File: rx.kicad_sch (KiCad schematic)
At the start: 49 parts, among them J5 SWH, J7 SMA, J9 SWH, T1 RF_BALUN, T1 RXIF_BALUN, U14 MAX2120, U16 DPDT

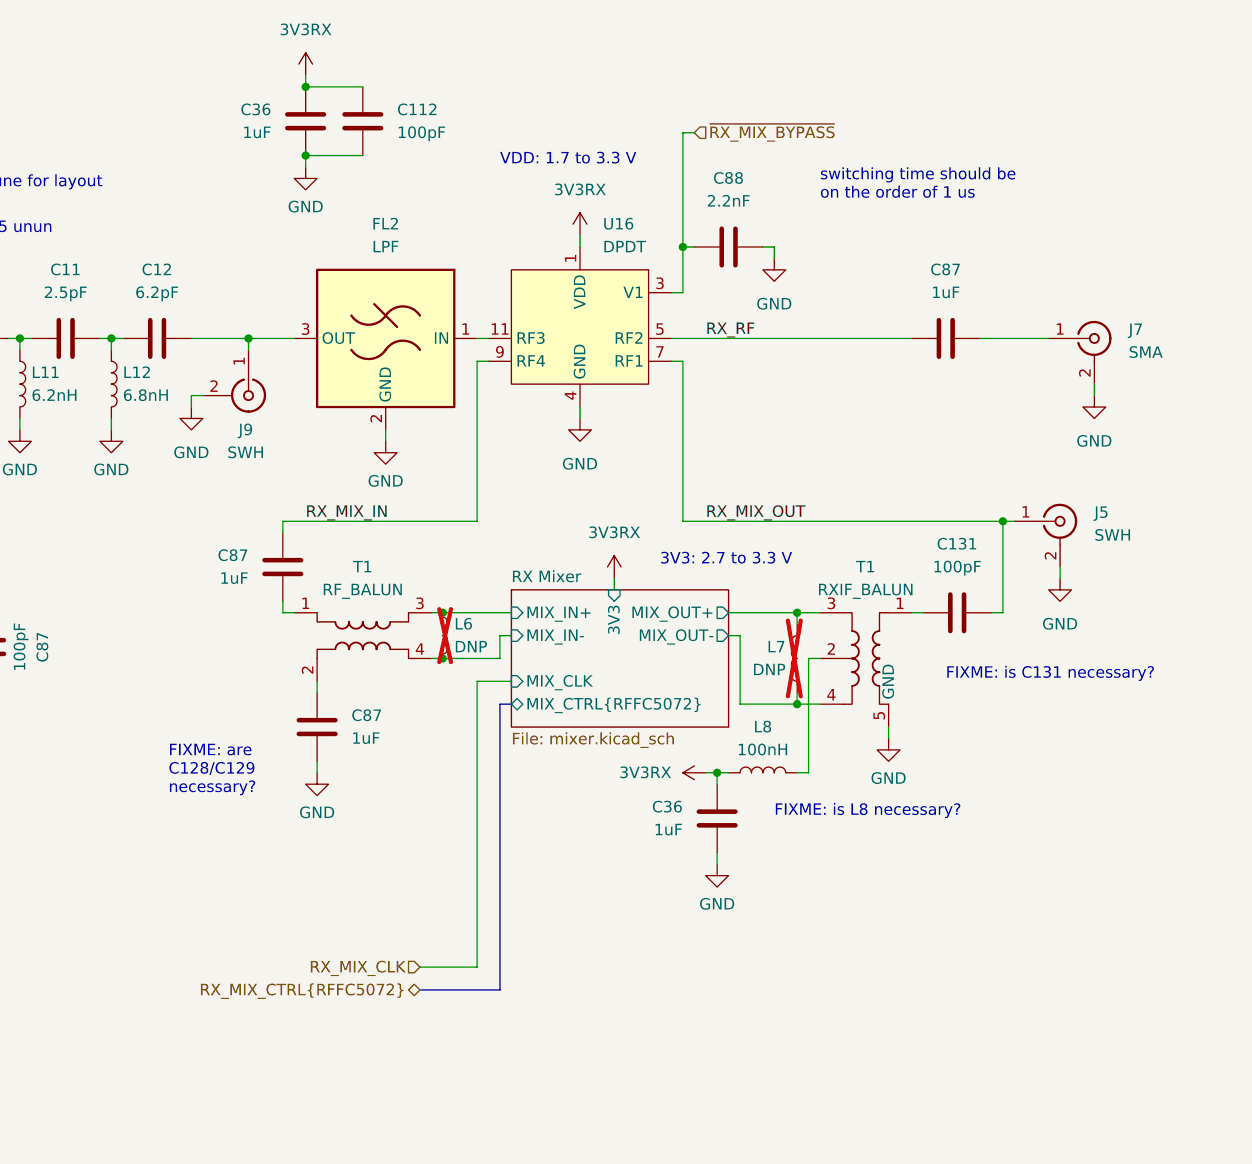
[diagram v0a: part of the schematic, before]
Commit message: add SWH connector symbols
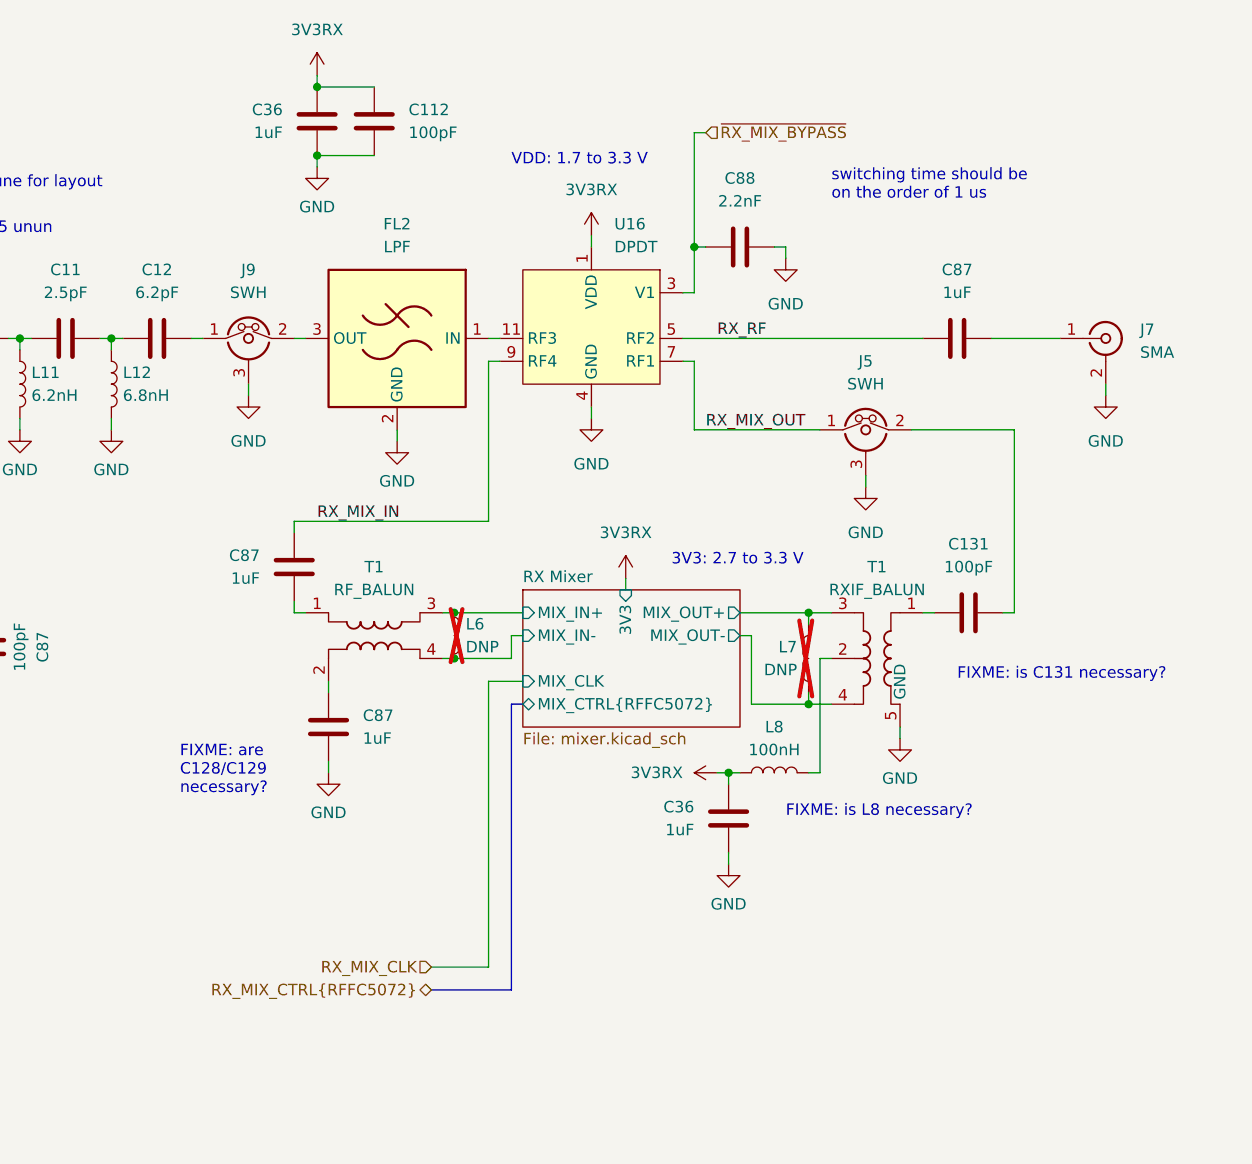
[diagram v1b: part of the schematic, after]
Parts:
- removed J5, J9: SWH, symbol Connector:Conn_Coaxial
- added J5, J9: SWH, symbol radio:Conn_Coaxial_MM8930-2620
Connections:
- net GND: now also J5.3 (Ext), J9.3 (Ext)
- net RX_MIX_OUT: now also J5.1 (C); no longer C131.1
- net at C12.2: now also J9.1 (C); no longer FL2.3 (OUT)
- new net: C131.1, J5.2 (R)
- new net: FL2.3 (OUT), J9.2 (R)
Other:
- moved on the sheet: C112, C131, C36, C87, C88, FL2, J7, L6, L7, L8, T1, U16
